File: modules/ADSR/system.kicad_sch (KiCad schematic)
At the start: 8 parts, among them J1 CardConnector, J2 ENV SELECT, J3 GATE SELECT, J4 EOS, J5 EGATE

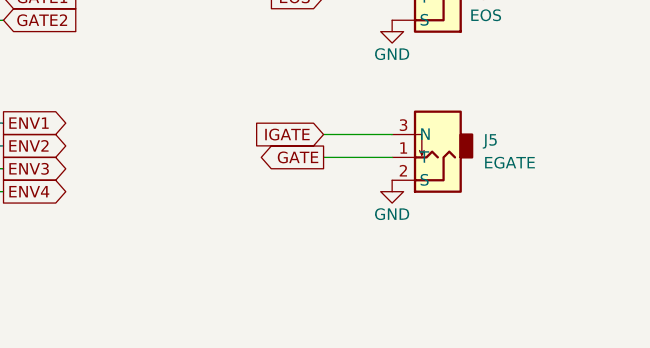
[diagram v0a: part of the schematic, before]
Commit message: adsr additions
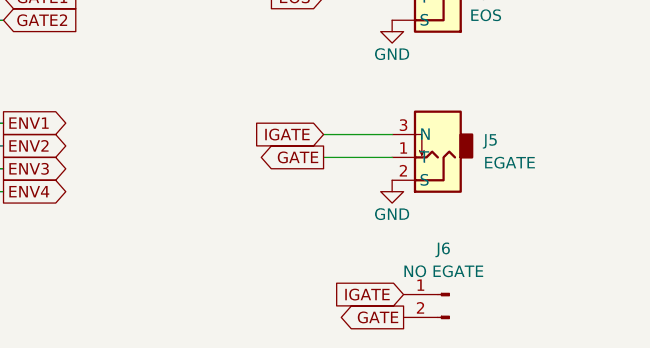
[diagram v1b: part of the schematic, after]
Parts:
- added J6: NO EGATE, FormantKO:Jumper_1x02, symbol FormantKO:Jumper_1x02
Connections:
- net GATE: now also J6.2 (Pin_2)
- net IGATE: now also J6.1 (Pin_1)
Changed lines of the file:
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@@
+		)
+	)
+	(global_label "GATE"
+		(shape output)
+		(at 161.29 137.16 180)
+		(fields_autoplaced yes)
+		(effects
+			(font
+				(size 1.27 1.27)
+			)
+			(justify right)
+		)
+		(property "Intersheetrefs" "${INTERSHEET_REFS}"
+			(at 153.7345 137.16 0)
+			(hide yes)
+			(show_name no)
+			(do_not_autoplace no)
+			(effects
+				(font
+					(size 1.27 1.27)
+				)
+				(justify right)
+			)
 		)
 	)
@@
 				)
 				(justify left)
+			)
+		)
+	)
+	(global_label "IGATE"
+		(shape input)
+		(at 161.29 134.62 180)
+		(fields_autoplaced yes)
+		(effects
+			(font
+				(size 1.27 1.27)
+			)
+			(justify right)
+		)
+		(property "Intersheetrefs" "${INTERSHEET_REFS}"
+			(at 153.1297 134.62 0)
+			(hide yes)
+			(show_name no)
+			(do_not_autoplace no)
+			(effects
+				(font
+					(size 1.27 1.27)
+				)
+				(justify right)
 			)
 		)
@@
 			)
 		)
+	)
+	(symbol
+		(lib_id "FormantKO:Jumper_1x02")
+		(at 166.37 134.62 0)
+		(mirror y)
+		(unit 1)
+		(body_style 1)
+		(exclude_from_sim no)
+		(in_bom yes)
+		(on_board yes)
+		(in_pos_files yes)
+		(dnp no)
+		(fields_autoplaced yes)
+		(property "Reference" "J6"
+			(at 165.735 129.54 0)
+			(show_name no)
+			(do_not_autoplace no)
+			(effects
+				(font
+					(size 1.27 1.27)
+				)
+			)
+		)
+		(property "Value" "NO EGATE"
+			(at 165.735 132.08 0)
+			(show_name no)
+			(do_not_autoplace no)
+			(effects
+				(font
+					(size 1.27 1.27)
+				)
+			)
+		)
+		(property "Footprint" "FormantKO:Jumper_1x02"
+			(at 166.37 134.62 0)
+			(hide yes)
+			(show_name no)
+			(do_not_autoplace no)
+			(effects
+				(font
+					(size 1.27 1.27)
+				)
+			)
+		)
+		(property "Datasheet" ""
+			(at 166.37 134.62 0)
+			(hide yes)
+			(show_name no)
+			(do_not_autoplace no)
+			(effects
+				(font
+					(size 1.27 1.27)
+				)
+			)
+		)
+		(property "Description" "Generic connector, single row, 01x02, script generated"
+			(at 166.37 134.62 0)
+			(hide yes)
+			(show_name no)
+			(do_not_autoplace no)
+			(effects
+				(font
+					(size 1.27 1.27)
+				)
+			)
+		)
+		(pin "1"
+		)
+		(pin "2"
+		)
+		(instances
+			(project "ADSR"
+				(path "/d2c8cc99-9c9f-481f-b15d-dad87d2b88db"
+					(reference "J6")
+					(unit 1)
+				)
+			)
+		)
